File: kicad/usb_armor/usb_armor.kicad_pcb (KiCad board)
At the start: 2 copper layers, 29 x 29 mm, 4 parts

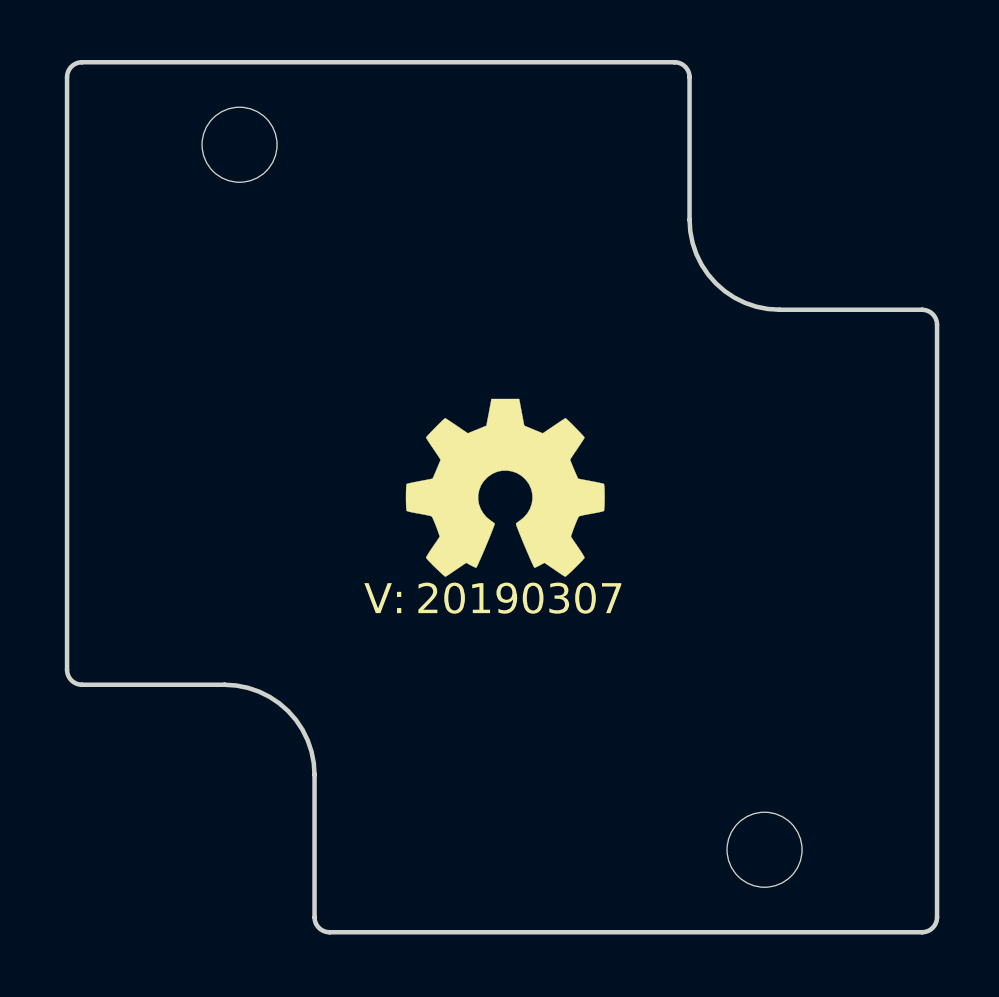
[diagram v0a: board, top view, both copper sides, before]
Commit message: initial schematic, routing, silk placement
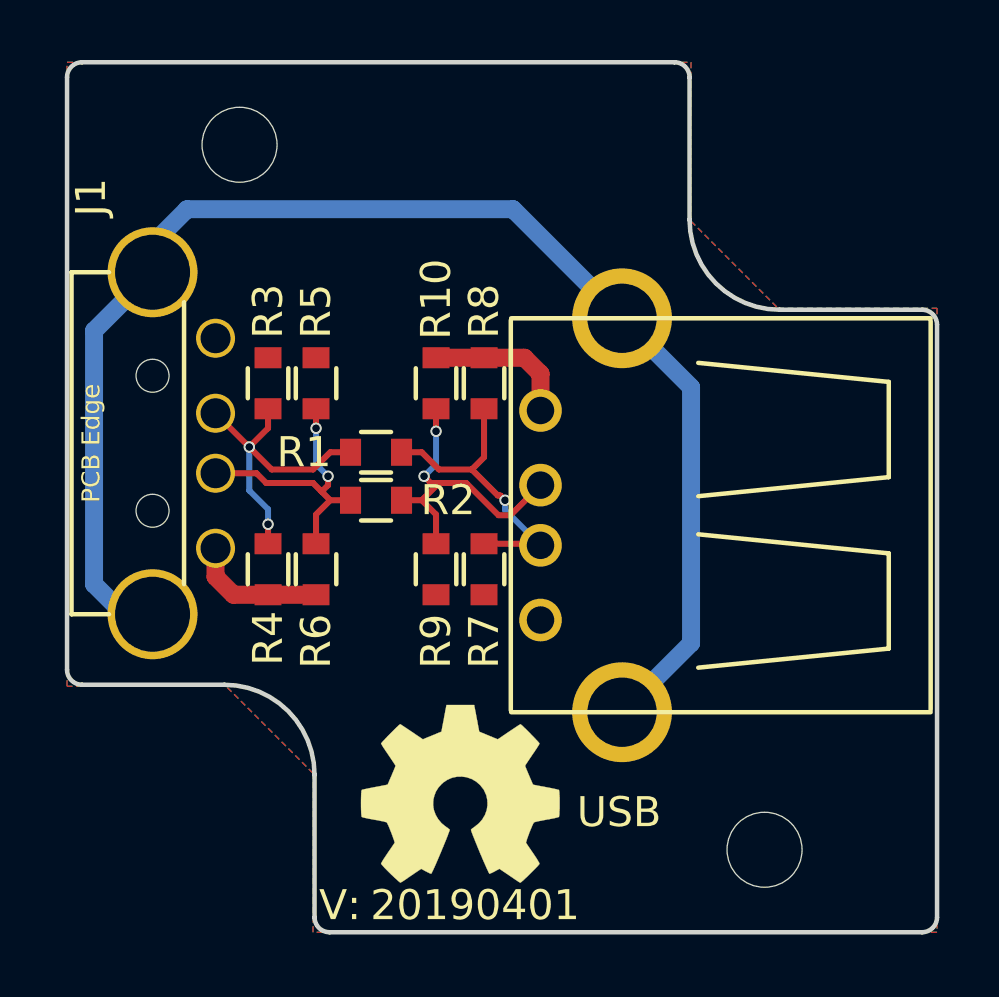
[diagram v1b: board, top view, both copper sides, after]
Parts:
- added J1: USB, SquantorUsb:USB_A-Plug-generic, F.Cu at (137.3, 99.5)
- added J2: USB, SquantorUsb:USB-A-TH, F.Cu at (151.9, 101.9)
- added R1: TBD, SquantorRcl:R_0603_hand, F.Cu at (143.7, 99.8)
- added R10: TBD, SquantorRcl:R_0603_hand, F.Cu at (145.7, 97.5)
- added R2: TBD, SquantorRcl:R_0603_hand, F.Cu at (143.7, 101.4)
- added R3: TBD, SquantorRcl:R_0603_hand, F.Cu at (140.1, 97.5)
- added R4: TBD, SquantorRcl:R_0603_hand, F.Cu at (140.1, 103.7)
- added R5: TBD, SquantorRcl:R_0603_hand, F.Cu at (141.7, 97.5)
- added R6: TBD, SquantorRcl:R_0603_hand, F.Cu at (141.7, 103.7)
- added R7: TBD, SquantorRcl:R_0603_hand, F.Cu at (147.3, 103.7)
- added R8: TBD, SquantorRcl:R_0603_hand, F.Cu at (147.3, 97.5)
- added R9: TBD, SquantorRcl:R_0603_hand, F.Cu at (145.7, 103.7)
- N2: value 20190307 -> 20190401
- moved N1 10.3 mm to (146.5, 111.2)
- moved N2 10.3 mm to (147.4, 115.0)
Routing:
- net /Shield: track 0.00 -> 47.2 mm
- net /IN_USB-D-: track 0.00 -> 10.5 mm, vias 0 -> 2
- net /OUT_USB-D+: track 0.00 -> 10.4 mm, vias 0 -> 2
- net /OUT_USB-D-: track 0.00 -> 10.2 mm, vias 0 -> 1
- net /IN_USB-D+: track 0.00 -> 9.54 mm, vias 0 -> 2
- net /GND: track 0.00 -> 9.48 mm
- added copper zone on B.Cu, net /GND
- added copper zone on F.Cu, net /VBUS
